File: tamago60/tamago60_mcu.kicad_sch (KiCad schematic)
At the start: 7 parts, among them J1 4105, J2 Cirque FFC, U1 kb2040

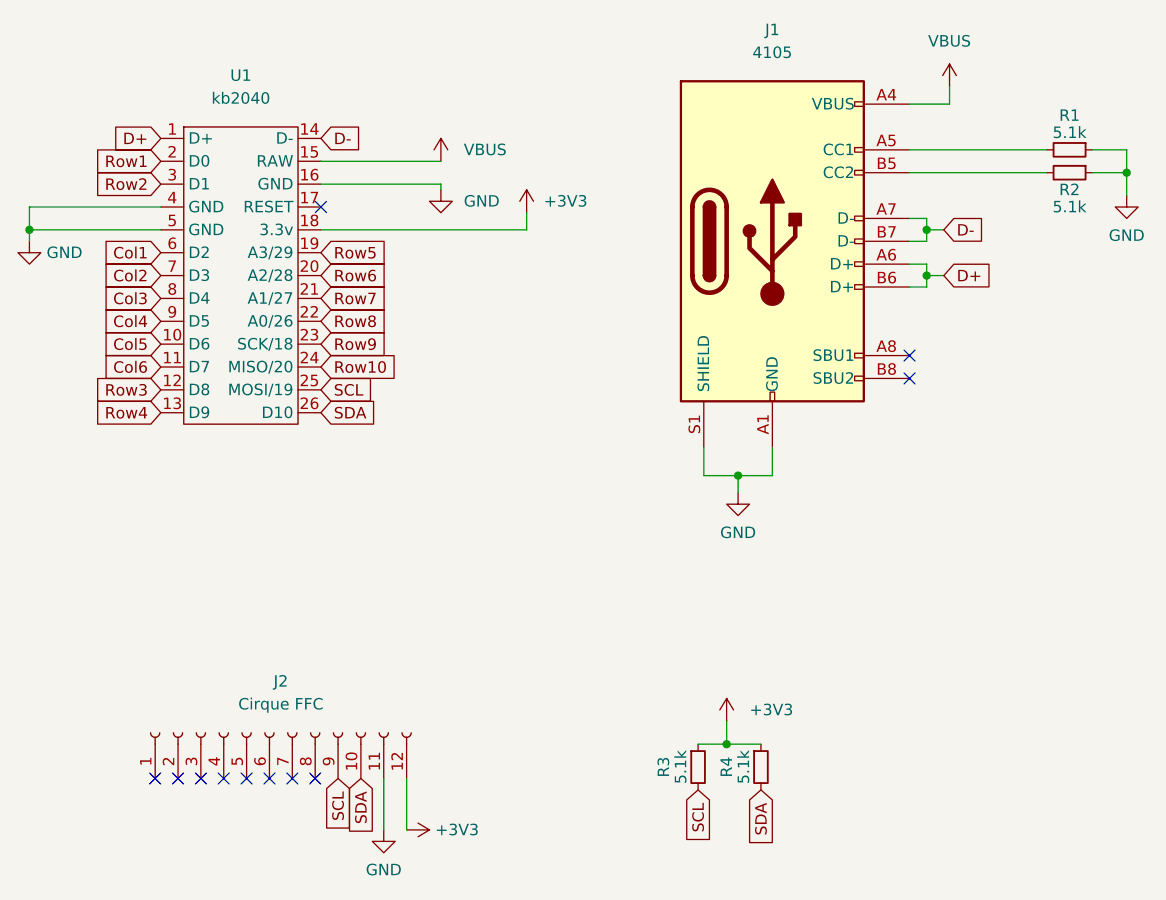
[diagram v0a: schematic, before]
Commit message: routing
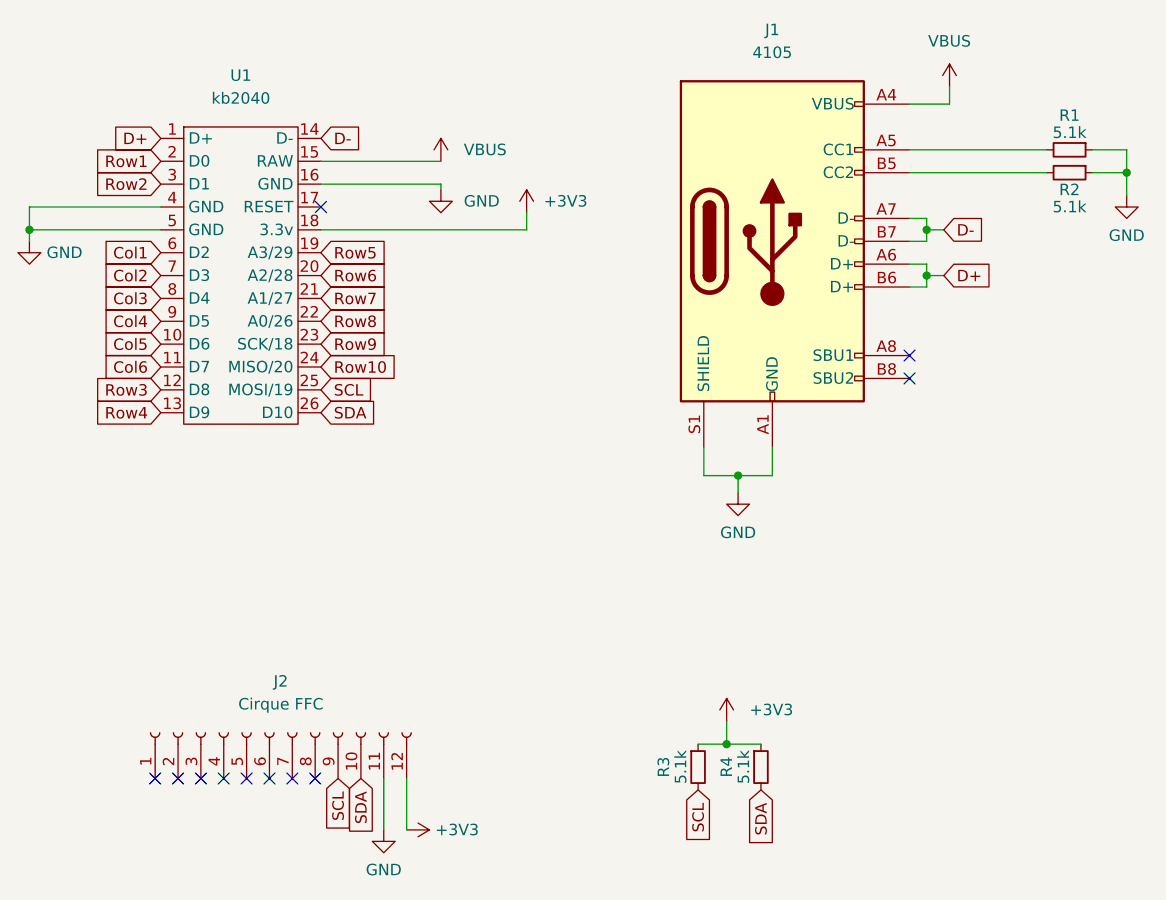
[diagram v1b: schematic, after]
